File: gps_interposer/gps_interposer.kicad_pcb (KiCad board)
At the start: 2 copper layers, 43 x 43.5 mm, 43 parts, among them J1 Module Connector, J2 Motherboard/Carrier Connector, J3 Ext VSYS, J4 GENERIC_3V0, J6 GENERIC_3V3, U1 SN74LVC1T45DBV, U2 SN74LVC1T45DBV, U3 RP20240-Zero, U4 SN74LVC1T45DBV, U5 SN74LVC1T45DBV, U6 SN74LVC1T45DBV, U7 SN74LVC1T45DBV

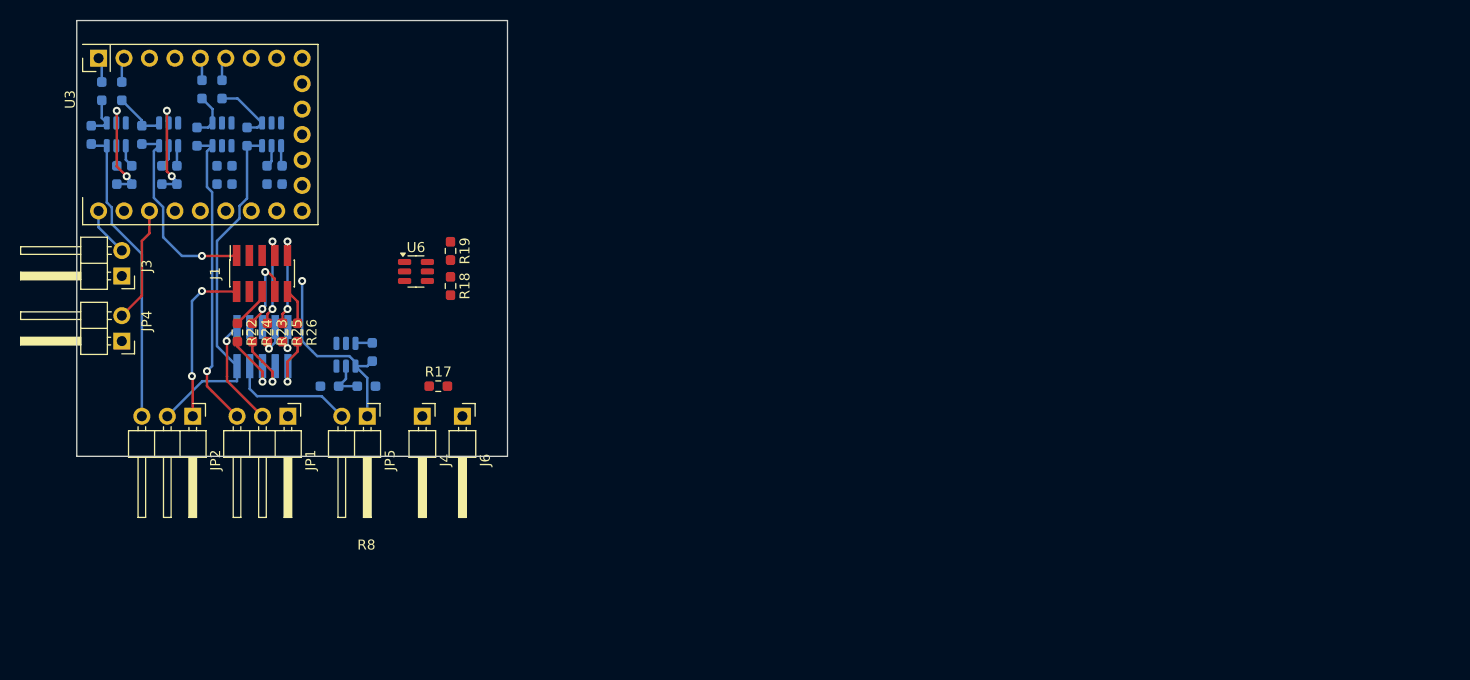
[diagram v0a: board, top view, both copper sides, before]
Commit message: PCB ready.
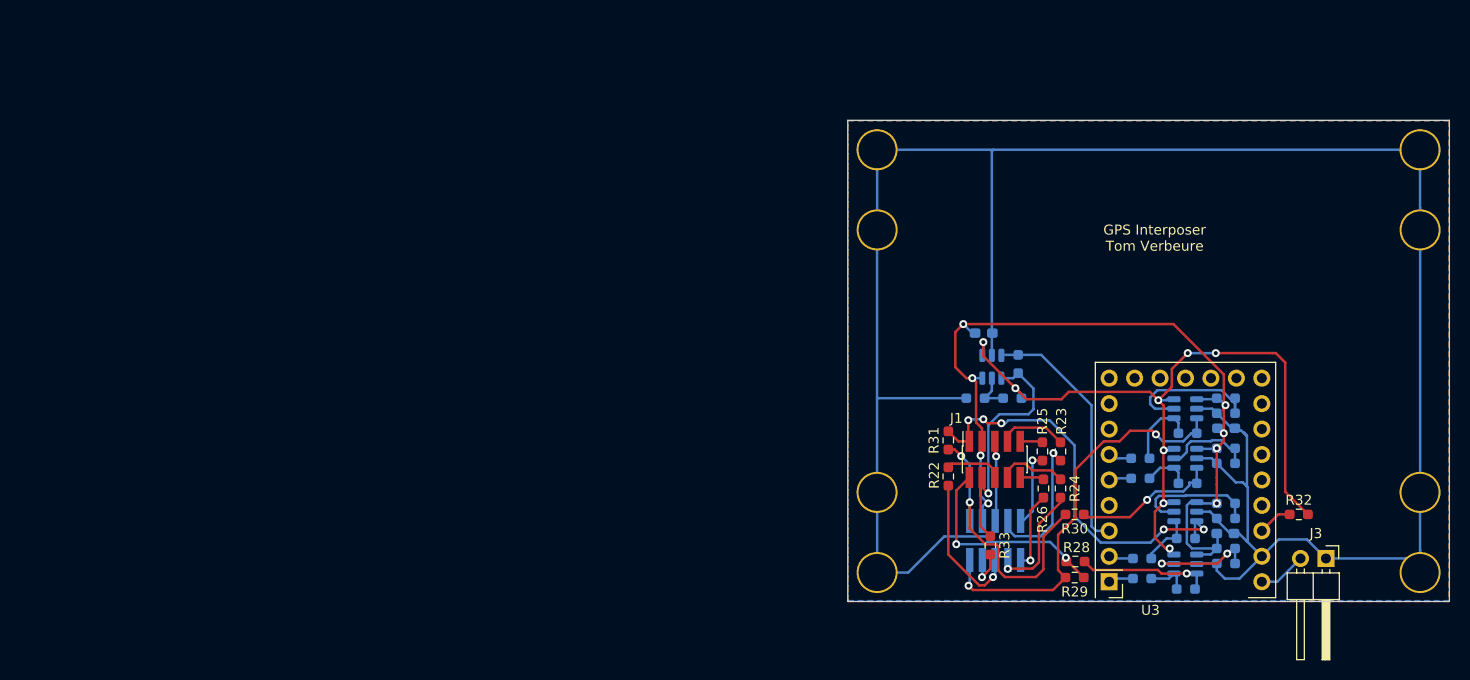
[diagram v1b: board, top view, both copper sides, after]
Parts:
- removed J4: GENERIC_3V0, Connector_PinHeader_2.54mm:PinHeader_1x01_P2.54mm_Horizontal
- removed J6: GENERIC_3V3, Connector_PinHeader_2.54mm:PinHeader_1x01_P2.54mm_Horizontal
- removed JP1: TXD Direct, Connector_PinHeader_2.54mm:PinHeader_1x03_P2.54mm_Horizontal
- removed JP2: RXD Direct, Connector_PinHeader_2.54mm:PinHeader_1x03_P2.54mm_Horizontal
- removed JP4: 3V3 Zero, Connector_PinHeader_2.54mm:PinHeader_1x02_P2.54mm_Horizontal
- removed JP5: 1PPS Direct, Connector_PinHeader_2.54mm:PinHeader_1x02_P2.54mm_Horizontal
- removed R17, R18: NC, Resistor_SMD:R_0603_1608Metric_Pad0.98x0.95mm_HandSolder
- removed R19: 1K, Resistor_SMD:R_0603_1608Metric_Pad0.98x0.95mm_HandSolder
- removed U6: SN74LVC1T45DBV, Package_TO_SOT_SMD:SOT-23-6
- added C1: 100n, Capacitor_SMD:C_0603_1608Metric_Pad1.08x0.95mm_HandSolder, B.Cu at (173.5, 88.2)
- added C2: 100n, Capacitor_SMD:C_0603_1608Metric_Pad1.08x0.95mm_HandSolder, B.Cu at (197.7, 108.2)
- added C4: 100n, Capacitor_SMD:C_0603_1608Metric_Pad1.08x0.95mm_HandSolder, B.Cu at (197.7, 97.7)
- added H1: MountingHole_Pad, Kicad_Personal:MountingHole_3.7mm_3.9mm_Pad_TopBottom, F.Cu at (217.1, 77.9)
- added H2: MountingHole_Pad, Kicad_Personal:MountingHole_3.7mm_3.9mm_Pad_TopBottom, F.Cu at (217.1, 112.1)
- added H3: MountingHole_Pad, Kicad_Personal:MountingHole_3.7mm_3.9mm_Pad_TopBottom, F.Cu at (162.9, 112.1)
- added H4: MountingHole_Pad, Kicad_Personal:MountingHole_3.7mm_3.9mm_Pad_TopBottom, F.Cu at (162.9, 77.9)
- added H5: MountingHole_Pad, Kicad_Personal:MountingHole_3.7mm_3.9mm_Pad_TopBottom, F.Cu at (162.9, 69.9)
- added H6: MountingHole_Pad, Kicad_Personal:MountingHole_3.7mm_3.9mm_Pad_TopBottom, F.Cu at (217.1, 69.9)
- added H7: MountingHole_Pad, Kicad_Personal:MountingHole_3.7mm_3.9mm_Pad_TopBottom, F.Cu at (217.1, 104.1)
- added H8: MountingHole_Pad, Kicad_Personal:MountingHole_3.7mm_3.9mm_Pad_TopBottom, F.Cu at (162.9, 104.1)
- added R28: NS, Resistor_SMD:R_0603_1608Metric_Pad0.98x0.95mm_HandSolder, F.Cu at (182.7, 111.0)
- added R29: 0, Resistor_SMD:R_0603_1608Metric_Pad0.98x0.95mm_HandSolder, F.Cu at (182.6, 112.6)
- added R30: NS, Resistor_SMD:R_0603_1608Metric_Pad0.98x0.95mm_HandSolder, F.Cu at (182.6, 106.3)
- added R31: 0, Resistor_SMD:R_0603_1608Metric_Pad0.98x0.95mm_HandSolder, F.Cu at (170.0, 98.9)
- added R32: 0, Resistor_SMD:R_0603_1608Metric_Pad0.98x0.95mm_HandSolder, F.Cu at (205.0, 106.3)
- added R33: 0, Resistor_SMD:R_0603_1608Metric_Pad0.98x0.95mm_HandSolder, F.Cu at (174.2, 109.4)
- R2, R5: value NC -> NS
- moved J3 123.5 mm to (207.7, 110.7), turned to -90 degrees
- moved R2 118.3 mm to (193.7, 113.8), turned to 180 degrees
- moved R6 117.3 mm to (197.7, 111.2), turned to 0 degrees
- moved R5 115.4 mm to (197.7, 109.7), turned to 180 degrees
- moved U1 115.0 mm to (193.7, 111.2), turned to 180 degrees
- moved R13 114.7 mm to (189.3, 112.7), turned to 0 degrees
- moved R14 112.0 mm to (189.3, 110.7), turned to 0 degrees
- moved R1 111.7 mm to (193.7, 108.7), turned to 0 degrees
- moved R3 111.6 mm to (197.7, 106.7), turned to 0 degrees
- moved R4 109.7 mm to (197.7, 105.2), turned to 180 degrees
- moved U2 108.3 mm to (193.7, 106.0), turned to 180 degrees
- moved R10 104.8 mm to (193.9, 103.2), turned to 180 degrees
- moved R12 104.7 mm to (197.7, 101.2), turned to 0 degrees
- moved U3 104.2 mm to (193.7, 102.9), turned to 180 degrees
- moved R11 102.9 mm to (197.7, 99.7), turned to 180 degrees
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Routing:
- net GND: track 6.49 -> 248.7 mm, vias 0 -> 1
- net +3V0: track 6.34 -> 86.6 mm, vias 0 -> 8
- net +3.3V: track 0.00 -> 76.8 mm, vias 0 -> 8
- net /1PPS_M_3V3: track 1.70 -> 25.1 mm
- net /TXD_M: track 20.0 -> 41.2 mm, vias 1 -> 5
- net /TXD_C: track 10.8 -> 28.5 mm, vias 1 -> 2
- net /RXD_M_3V0: track 30.1 -> 13.3 mm, vias 0 -> 1
- net /TXD_C_3V0: track 30.4 -> 14.6 mm
- net Net-(U7-DIR): track 0.00 -> 15.9 mm
- net /RSVD7_C: track 3.19 -> 14.3 mm
- net Net-(U5-DIR): track 0.00 -> 9.07 mm
- net /1PPS_C: track 12.6 -> 4.34 mm, vias 0 -> 1
- net /BATT_C: track 6.59 -> 14.7 mm
- net Net-(U3-3V3): track 11.6 -> 3.45 mm
- net /ANT_BIAS_M: track 9.78 -> 2.26 mm, vias 2 -> 0
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- added copper zone on F.Cu, net +3V0
- added copper zone on B.Cu, net GND
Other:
- board size 43 x 43.5 mm -> 60.1 x 48 mm
- board text added: "GPS Interposer Tom Verbeure"
